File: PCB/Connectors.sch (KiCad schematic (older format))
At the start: 17 parts, among them J1 S2B-PH-SM4-TB, J10 DNP, J11 DNP, J12 DNP, J2 TRANSDUCER, J3 DNP, J4 PH1-08-UA, J5 DNP, J6 DNP, J7 DNP, J8 PH1-08-UA, J9 DNP

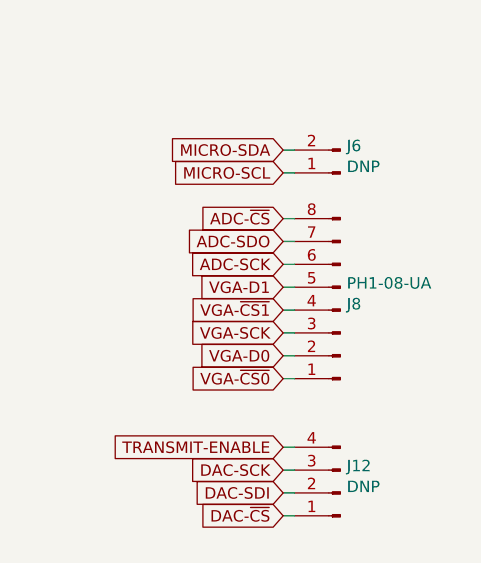
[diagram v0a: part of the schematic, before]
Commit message: Tiny fixes to the schematic
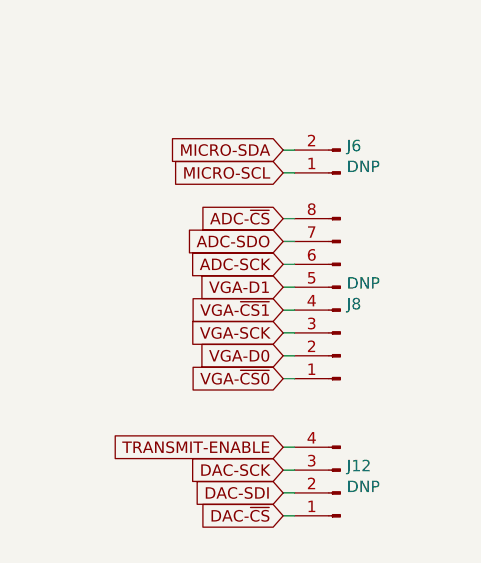
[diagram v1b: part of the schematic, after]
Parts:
- J8: value PH1-08-UA -> DNP
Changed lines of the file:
@@
 P 9050 5200
 F 0 "J8" H 9022 5174 50  0000 R CNN
-F 1 "PH1-08-UA" H 9022 5083 50  0000 R CNN
+F 1 "DNP" H 9022 5083 50  0000 R CNN
 F 2 "Pin_Headers:Pin_Header_Straight_1x08_Pitch2.54mm" H 9050 5200 50  0001 C CNN
 F 3 "https://www.digikey.ca/product-detail/en/adam-tech/PH1-08-UA/2057-PH1-08-UA-ND/9830442" H 9050 5200 50  0001 C CNN
